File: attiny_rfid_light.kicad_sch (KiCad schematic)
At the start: 28 parts, among them IC1 EM4095, J1 Conn_01x16_Male, U1 ESP32-WROOM-32, U2 NCP1117-3.3_SOT223

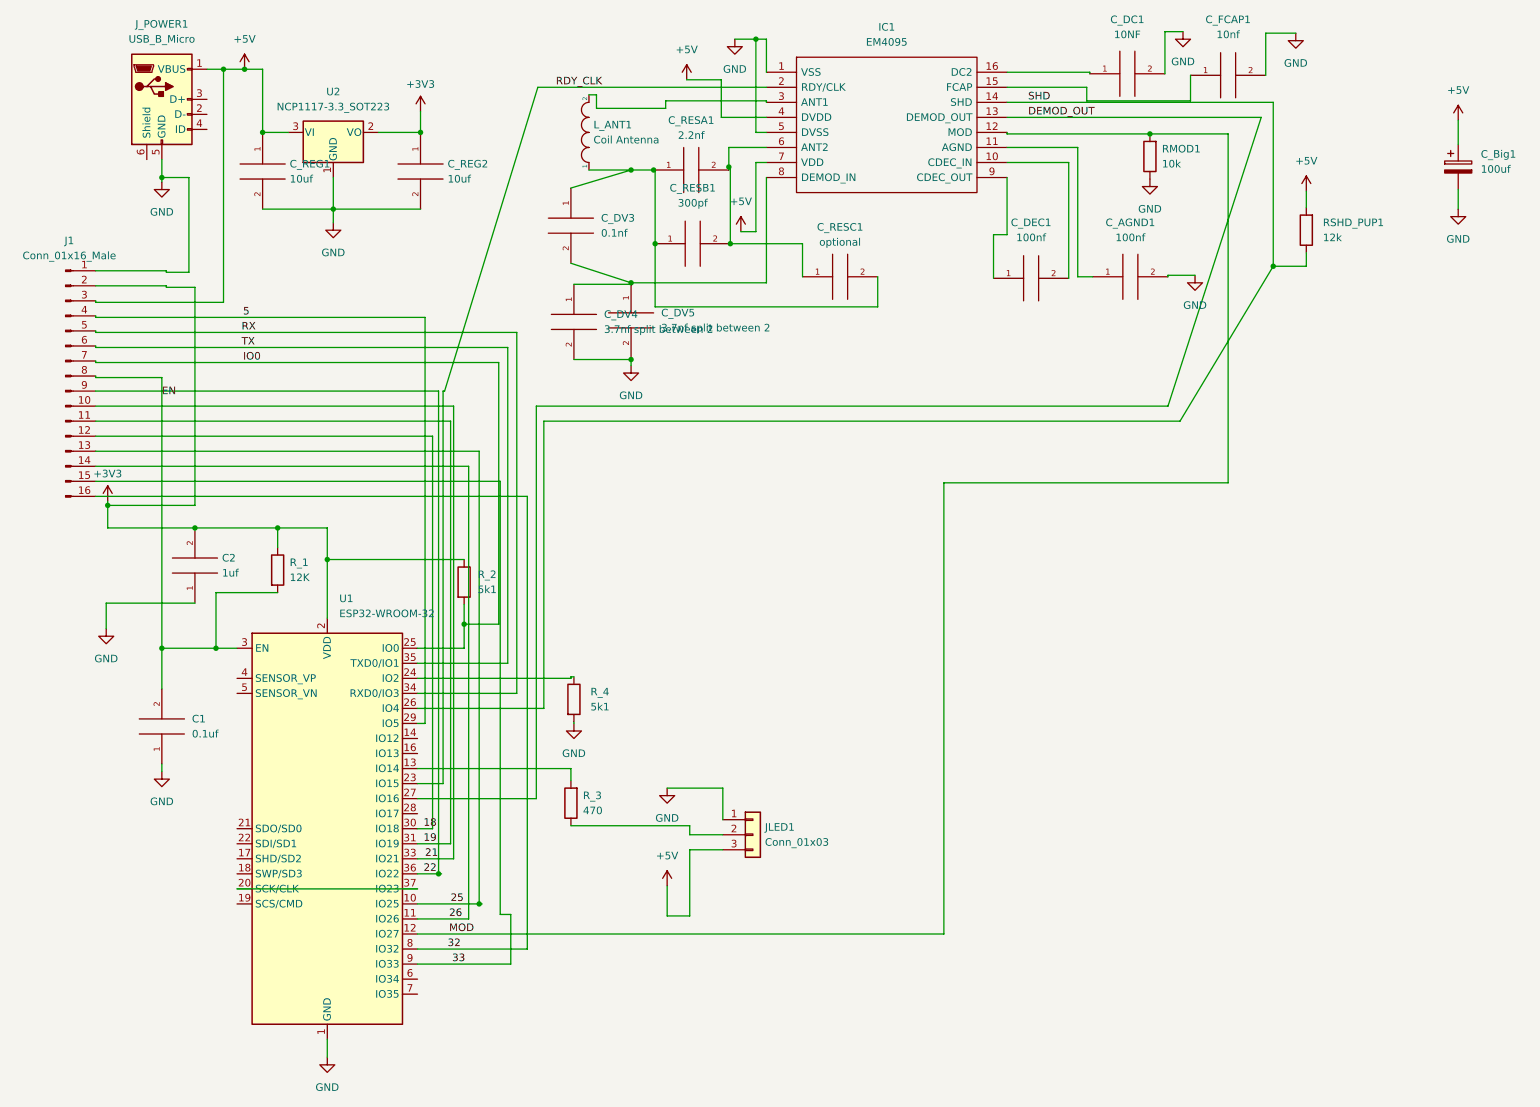
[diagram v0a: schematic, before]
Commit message: v5
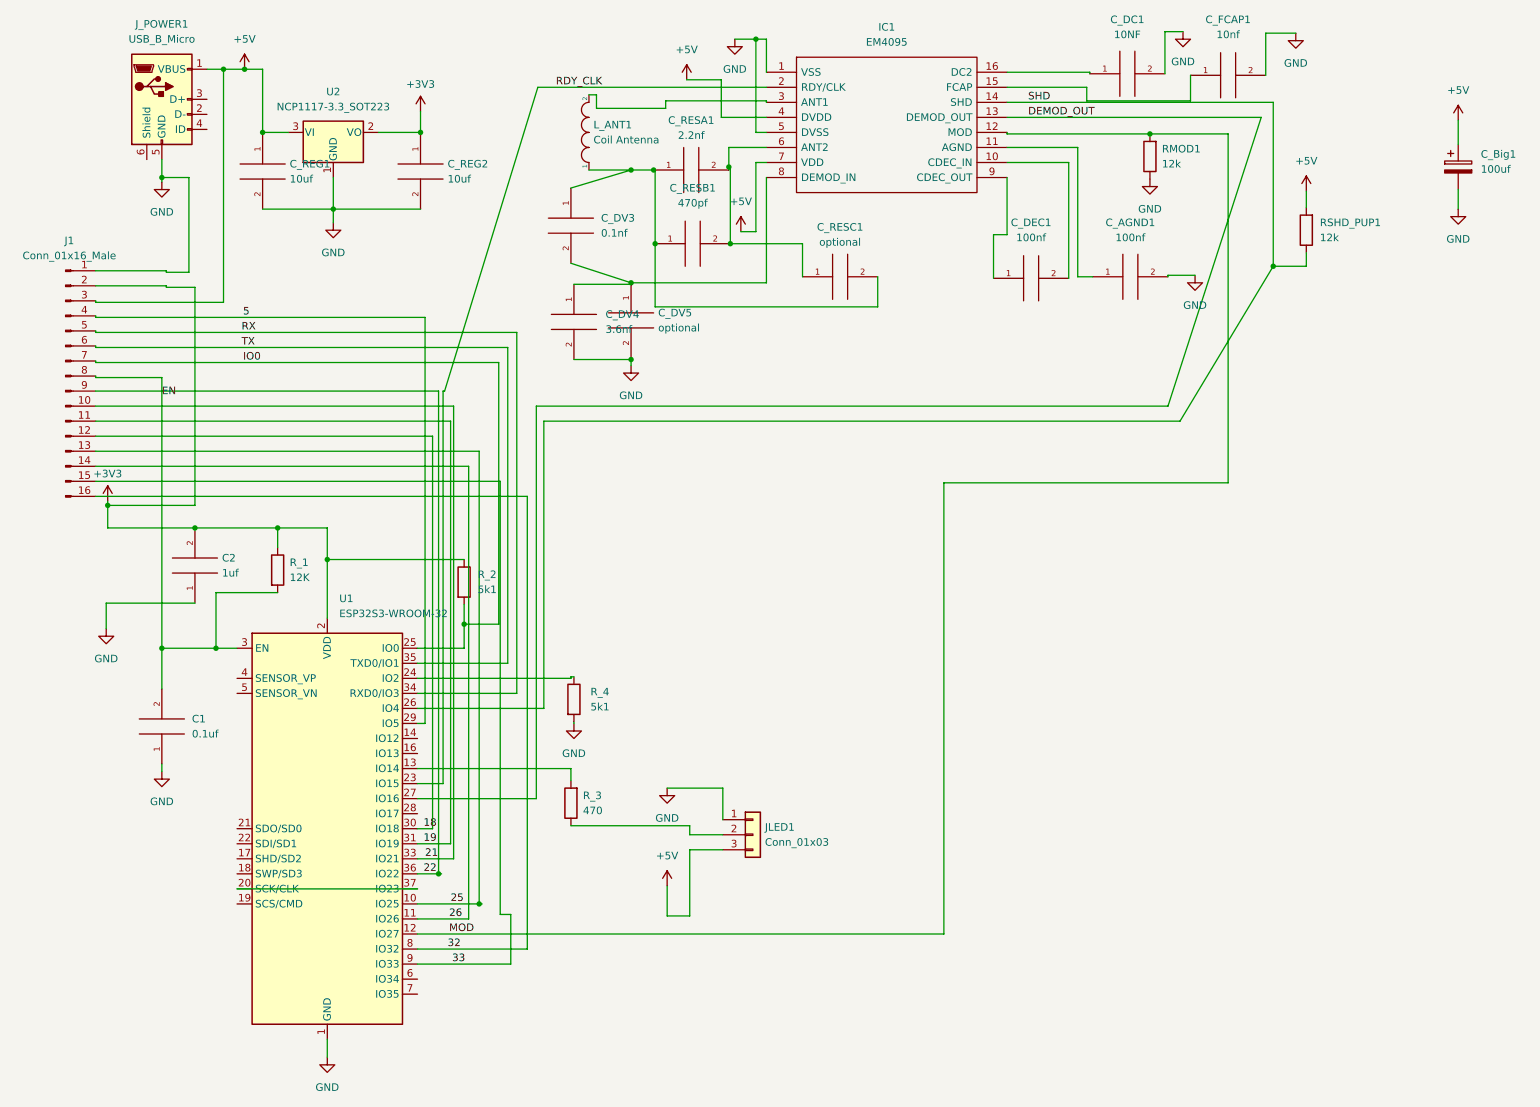
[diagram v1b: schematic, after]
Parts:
- C_DV4: value 3.7nf split between 2 -> 3.6nf
- C_DV5: value 3.7nf split between 2 -> optional
- C_RESB1: value 300pf -> 470pf
- RMOD1: value 10k -> 12k
- U1: value ESP32-WROOM-32 -> ESP32S3-WROOM-32
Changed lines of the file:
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@@
   (symbol (lib_id "pspice:C") (at 109.728 65.532 0) (unit 1)
     (in_bom yes) (on_board yes) (fields_autoplaced)
-    (property "Reference" "C_DV5" (id 0) (at 114.808 64.2619 0)
-      (effects (font (size 1.27 1.27)) (justify left))
-    )
-    (property "Value" "3.7nf split between 2" (id 1) (at 114.808 66.8019 0)
+    (property "Reference" "C_DV5" (id 0) (at 114.3 64.2619 0)
+      (effects (font (size 1.27 1.27)) (justify left))
+    )
+    (property "Value" "optional" (id 1) (at 114.3 66.8019 0)
       (effects (font (size 1.27 1.27)) (justify left))
     )
@@
   (symbol (lib_id "power:GND") (at 197.358 41.656 0) (unit 1)
     (in_bom yes) (on_board yes) (fields_autoplaced)
-    (property "Reference" "#PWR?" (id 0) (at 197.358 48.006 0)
+    (property "Reference" "#PWR0101" (id 0) (at 197.358 48.006 0)
       (effects (font (size 1.27 1.27)) hide)
     )
@@
   (symbol (lib_id "Device:R") (at 223.774 50.292 180) (unit 1)
     (in_bom yes) (on_board yes) (fields_autoplaced)
-    (property "Reference" "RSHD_PUP1" (id 0) (at 226.568 49.0219 0)
-      (effects (font (size 1.27 1.27)) (justify right))
-    )
-    (property "Value" "12k" (id 1) (at 226.568 51.5619 0)
+    (property "Reference" "RSHD_PUP1" (id 0) (at 226.06 49.0219 0)
+      (effects (font (size 1.27 1.27)) (justify right))
+    )
+    (property "Value" "12k" (id 1) (at 226.06 51.5619 0)
       (effects (font (size 1.27 1.27)) (justify right))
     )
@@
     (in_bom yes) (on_board yes) (fields_autoplaced)
     (property "Reference" "C_RESB1" (id 0) (at 120.142 43.18 90))
-    (property "Value" "300pf" (id 1) (at 120.142 45.72 90))
+    (property "Value" "470pf" (id 1) (at 120.142 45.72 90))
     (property "Footprint" "Capacitor_SMD:C_0805_2012Metric_Pad1.18x1.45mm_HandSolder" (id 2) (at 120.142 52.578 0)
       (effects (font (size 1.27 1.27)) hide)
@@
       (effects (font (size 1.27 1.27)) (justify right))
     )
-    (property "Value" "10k" (id 1) (at 199.39 39.1159 0)
+    (property "Value" "12k" (id 1) (at 199.39 39.1159 0)
       (effects (font (size 1.27 1.27)) (justify right))
     )
@@
       (effects (font (size 1.27 1.27)) (justify left))
     )
-    (property "Value" "ESP32-WROOM-32" (id 1) (at 60.4394 115.062 0)
+    (property "Value" "ESP32S3-WROOM-32" (id 1) (at 60.4394 115.062 0)
       (effects (font (size 1.27 1.27)) (justify left))
     )
@@
   (symbol (lib_id "pspice:C") (at 100.076 65.786 0) (unit 1)
     (in_bom yes) (on_board yes) (fields_autoplaced)
-    (property "Reference" "C_DV4" (id 0) (at 105.156 64.5159 0)
-      (effects (font (size 1.27 1.27)) (justify left))
-    )
-    (property "Value" "3.7nf split between 2" (id 1) (at 105.156 67.0559 0)
+    (property "Reference" "C_DV4" (id 0) (at 105.41 64.5159 0)
+      (effects (font (size 1.27 1.27)) (justify left))
+    )
+    (property "Value" "3.6nf" (id 1) (at 105.41 67.0559 0)
       (effects (font (size 1.27 1.27)) (justify left))
     )
@@
     )
     (path "/22d7c125-9cf1-4deb-b5d5-b51921c98da9"
-      (reference "#PWR?") (unit 1) (value "GND") (footprint "")
+      (reference "#PWR0101") (unit 1) (value "GND") (footprint "")
     )
     (path "/64dd7740-0c72-400b-88d0-286b4c64ef49"
@@
     )
     (path "/fd781061-b786-4aa7-81c8-507570ec21b2"
-      (reference "C_DV4") (unit 1) (value "3.7nf split between 2") (footprint "Capacitor_SMD:C_0805_2012Metric_Pad1.18x1.45mm_HandSolder")
+      (reference "C_DV4") (unit 1) (value "3.6nf") (footprint "Capacitor_SMD:C_0805_2012Metric_Pad1.18x1.45mm_HandSolder")
     )
     (path "/0970727f-11dd-473f-b585-f40294eee11b"
-      (reference "C_DV5") (unit 1) (value "3.7nf split between 2") (footprint "Capacitor_SMD:C_0805_2012Metric_Pad1.18x1.45mm_HandSolder")
+      (reference "C_DV5") (unit 1) (value "optional") (footprint "Capacitor_SMD:C_0805_2012Metric_Pad1.18x1.45mm_HandSolder")
     )
     (path "/5fade6ac-277b-43df-8e3a-ea7ae9efe0a9"
@@
     )
     (path "/9f822722-8d50-42f5-a09c-1e6f990511b7"
-      (reference "C_RESB1") (unit 1) (value "300pf") (footprint "Capacitor_SMD:C_0805_2012Metric_Pad1.18x1.45mm_HandSolder")
+      (reference "C_RESB1") (unit 1) (value "470pf") (footprint "Capacitor_SMD:C_0805_2012Metric_Pad1.18x1.45mm_HandSolder")
     )
     (path "/a97e32ce-d185-4613-bc22-b319deb2b8c6"
@@
     )
     (path "/b5d9e330-bd91-4c98-8aec-669ce9e63550"
-      (reference "RMOD1") (unit 1) (value "10k") (footprint "Resistor_SMD:R_0805_2012Metric_Pad1.20x1.40mm_HandSolder")
+      (reference "RMOD1") (unit 1) (value "12k") (footprint "Resistor_SMD:R_0805_2012Metric_Pad1.20x1.40mm_HandSolder")
     )
     (path "/81c65984-9f9d-492c-82f9-bbe24b88ebc2"
@@
     )
     (path "/dd8613f5-26c5-442c-934d-db0fe188f421"
-      (reference "U1") (unit 1) (value "ESP32-WROOM-32") (footprint "RF_Module:ESP32-WROOM-32")
+      (reference "U1") (unit 1) (value "ESP32S3-WROOM-32") (footprint "RF_Module:ESP32-WROOM-32")
     )
     (path "/d2fc0903-7aa6-406c-9d43-15f34b985517"
